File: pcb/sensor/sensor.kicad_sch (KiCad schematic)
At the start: 53 parts, among them J3 sig_in, J4 sig_out, J7 Conn_02x02_Counter_Clockwise, SW2 SW_SPST, U1 SIT1042AQT/3, U2 HX711, U5 LMR16030SDDAR, U8 LMR16030SDDAR, U9 LMR16030SDDAR

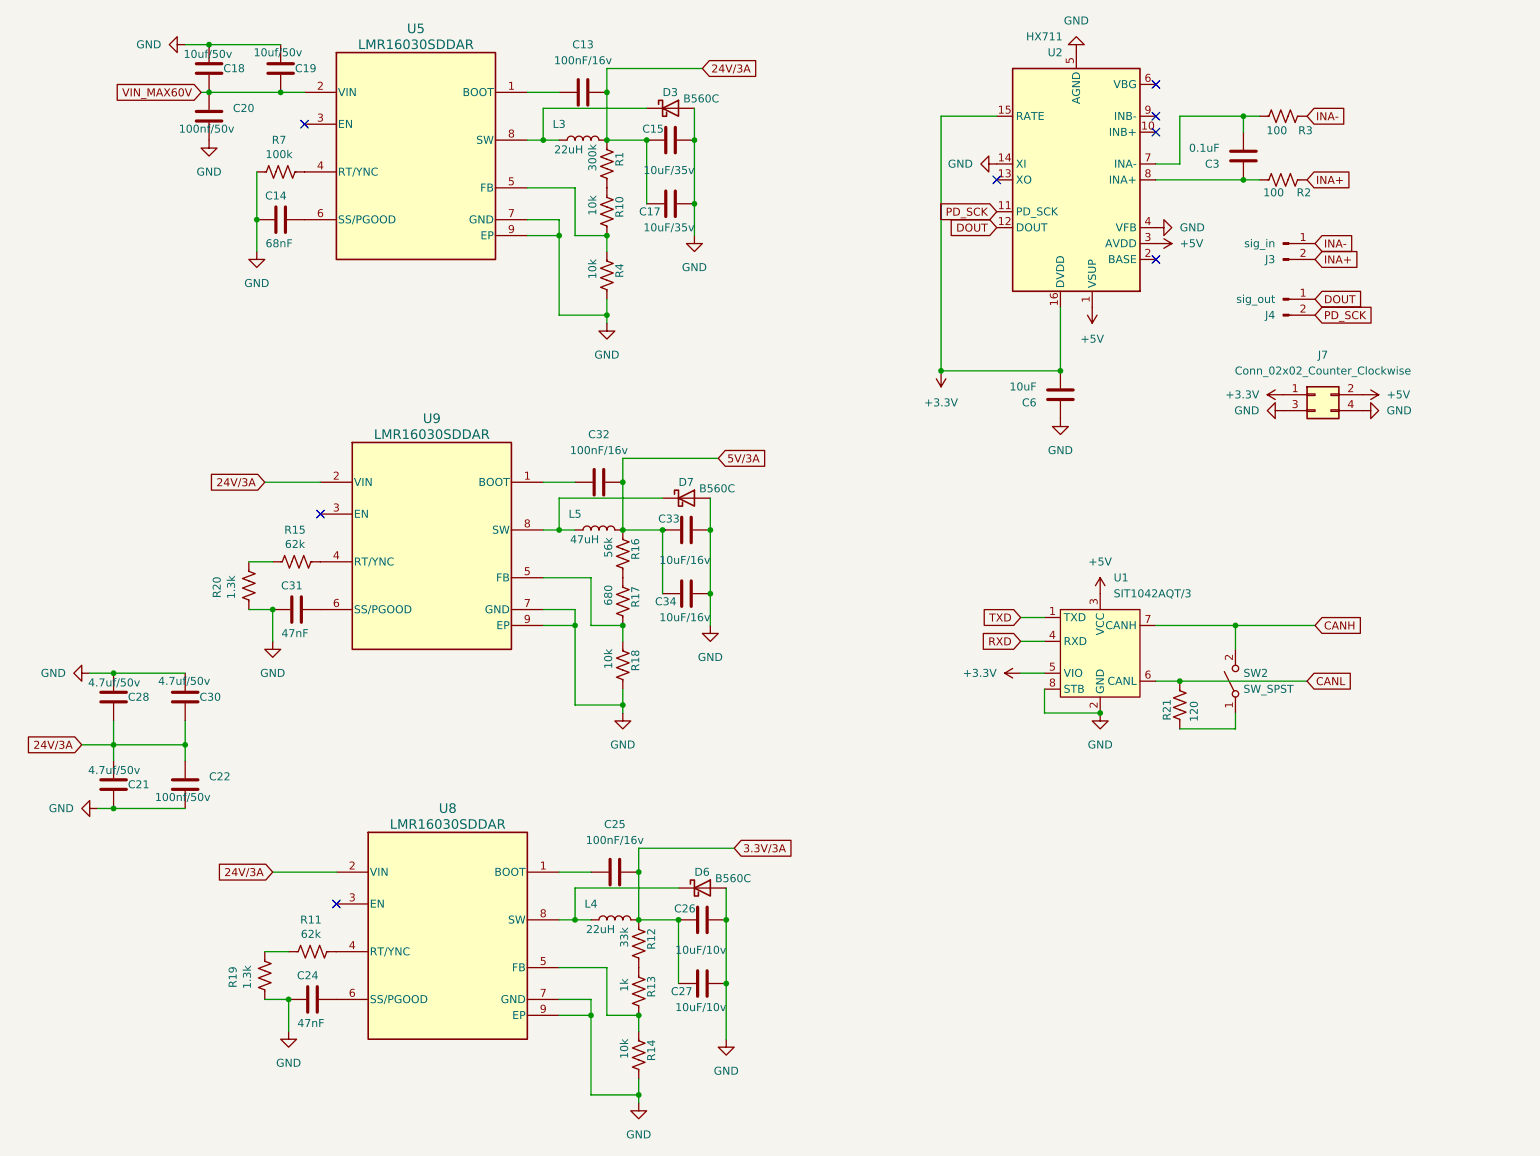
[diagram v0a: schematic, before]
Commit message: feat: update
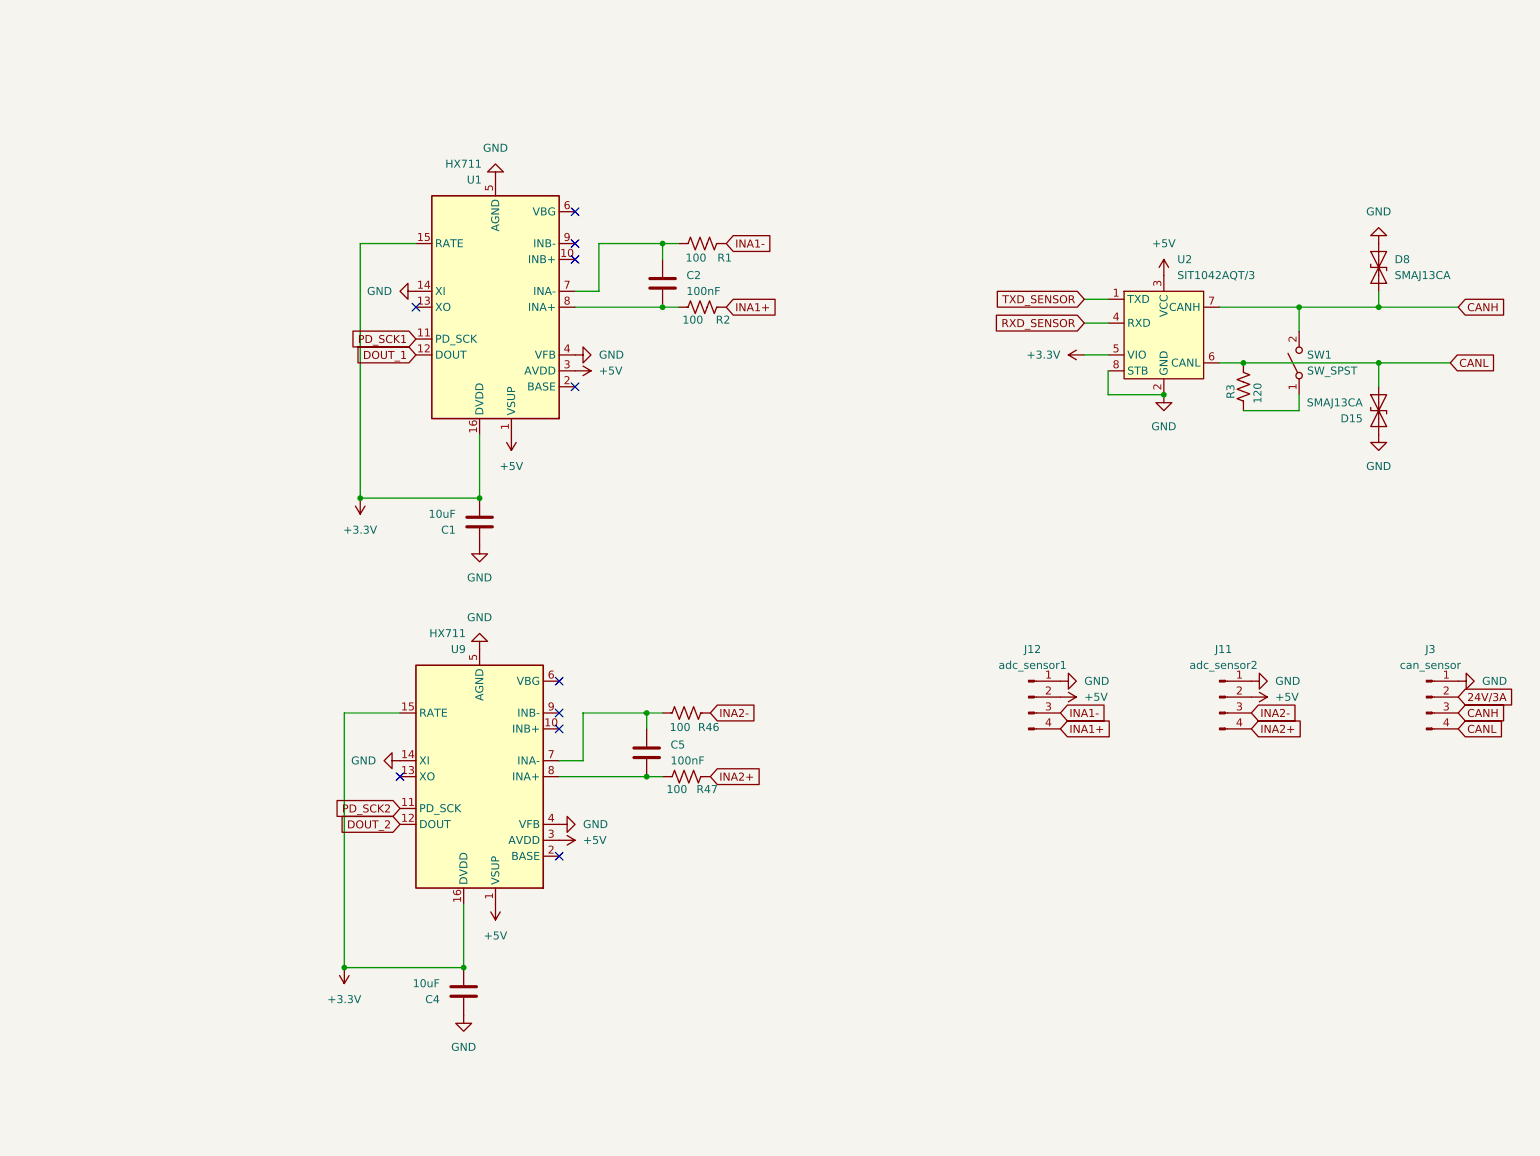
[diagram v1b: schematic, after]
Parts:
- removed C13, C25, C32: 100nF/16v, Capacitor_SMD:C_0603_1608Metric, symbol Device:C
- removed C14: 68nF, Capacitor_SMD:C_0603_1608Metric, symbol Device:C
- removed C15, C17: 10uF/35v, Capacitor_SMD:C_1210_3225Metric, symbol Device:C
- removed C18, C19: 10uf/50v, Capacitor_SMD:C_1210_3225Metric, symbol Device:C
- removed C20, C22: 100nf/50v, Capacitor_SMD:C_0603_1608Metric, symbol Device:C
- removed C21, C28, C30: 4.7uf/50v, Capacitor_SMD:C_1206_3216Metric, symbol Device:C
- removed C24, C31: 47nF, Capacitor_SMD:C_0603_1608Metric, symbol Device:C
- removed C26, C27: 10uF/10v, Capacitor_SMD:C_0603_1608Metric, symbol Device:C
- removed C33, C34: 10uF/16v, Capacitor_SMD:C_1210_3225Metric, symbol Device:C
- removed D3, D6, D7: B560C, Diode_SMD:D_SMC, symbol Device:D_Schottky
- removed J3: sig_in, Connector_PinHeader_2.54mm:PinHeader_1x02_P2.54mm_Vertical, symbol Connector:Conn_01x02_Pin
- removed J4: sig_out, Connector_PinHeader_2.54mm:PinHeader_1x02_P2.54mm_Vertical, symbol Connector:Conn_01x02_Pin
- removed J7: Conn_02x02_Counter_Clockwise, Connector_PinHeader_2.54mm:PinHeader_2x02_P2.54mm_Vertical, symbol Connector_Generic:Conn_02x02_Odd_Even
- removed L3, L4: 22uH, Inductor_SMD:L_TDK_SLF12565, symbol Device:L
- removed L5: 47uH, Inductor_SMD:L_TDK_SLF12565, symbol Device:L
- removed R1: 300k, Resistor_SMD:R_0603_1608Metric, symbol Device:R_US
- removed R10, R14, R18, R4: 10k, Resistor_SMD:R_0603_1608Metric, symbol Device:R_US
- removed R11, R15: 62k, Resistor_SMD:R_0603_1608Metric, symbol Device:R_US
- removed R12: 33k, Resistor_SMD:R_0603_1608Metric, symbol Device:R_US
- removed R13: 1k, Resistor_SMD:R_0603_1608Metric, symbol Device:R_US
- removed R16: 56k, Resistor_SMD:R_0603_1608Metric, symbol Device:R_US
- removed R17: 680, Resistor_SMD:R_0603_1608Metric, symbol Device:R_US
- removed R19, R20: 1.3k, Resistor_SMD:R_0603_1608Metric, symbol Device:R_US
- removed R7: 100k, Resistor_SMD:R_0603_1608Metric, symbol Device:R_US
- removed U5, U8, U9: LMR16030SDDAR, Package_SO:TI_SO-PowerPAD-8_ThermalVias, symbol 2025-01-08_11-11-09:LMR16030SDDAR
- added C4: 10uF, Capacitor_SMD:C_0603_1608Metric, symbol Device:C
- added C5: 100nF, Capacitor_SMD:C_0603_1608Metric, symbol Device:C
- added D15, D8: SMAJ13CA, Diode_SMD:D_SMA, symbol Diode:SMAJ13CA
- added J11: adc_sensor2, TerminalBlock:TerminalBlock_MaiXu_MX126-5.0-04P_1x04_P5.00mm, symbol Connector:Conn_01x04_Pin
- added J12: adc_sensor1, TerminalBlock:TerminalBlock_MaiXu_MX126-5.0-04P_1x04_P5.00mm, symbol Connector:Conn_01x04_Pin
- added J3: can_sensor, TerminalBlock:TerminalBlock_MaiXu_MX126-5.0-04P_1x04_P5.00mm, symbol Connector:Conn_01x04_Pin
- added R46, R47: 100, Resistor_SMD:R_0603_1608Metric, symbol Device:R_US
- added U9: HX711, Package_SO:SOP-16_3.9x9.9mm_P1.27mm, symbol Analog_ADC:HX711
- C2: renamed from C3; value 0.1uF -> 100nF
- renumbered C6 to C1, R3 to R1, R21 to R3, SW2 to SW1, U2 to U1, U1 to U2
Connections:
- net +3.3V: now also C4.2, U9.15 (RATE), U9.16 (DVDD)
- net +5V: now also J11.2 (Pin_2), J12.2 (Pin_2), U9.1 (VSUP), U9.3 (AVDD)
- net 24V/3A: now also J3.2 (Pin_2)
- net CANH: now also D8.1 (A1), J3.3 (Pin_3)
- net CANL: now also D15.1 (A1), J3.4 (Pin_4)
- net GND: now also C4.1, D15.2 (A2), D8.2 (A2), J11.1 (Pin_1), J12.1 (Pin_1), J3.1 (Pin_1), U9.14 (XI), U9.4 (VFB), U9.5 (AGND)
- net DOUT renamed DOUT_1
- net INA+ renamed INA1+
- net INA1+: now also J12.4 (Pin_4)
- net INA- renamed INA1-
- net INA1-: now also J12.3 (Pin_3)
- net PD_SCK renamed PD_SCK1
- net RXD renamed RXD_SENSOR
- net TXD renamed TXD_SENSOR
- new net: C5.1, R47.1, U9.8 (INA+)
- new net: C5.2, R46.1, U9.7 (INA-)
- new net DOUT_2: U9.12 (DOUT)
- new net INA2+: J11.4 (Pin_4), R47.2
- new net INA2-: J11.3 (Pin_3), R46.2
- new net PD_SCK2: U9.11 (PD_SCK)
- no-connect marks 8 -> 10
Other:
- moved on the sheet: C1, C2, R1, R2, R3, SW1, U1, U2

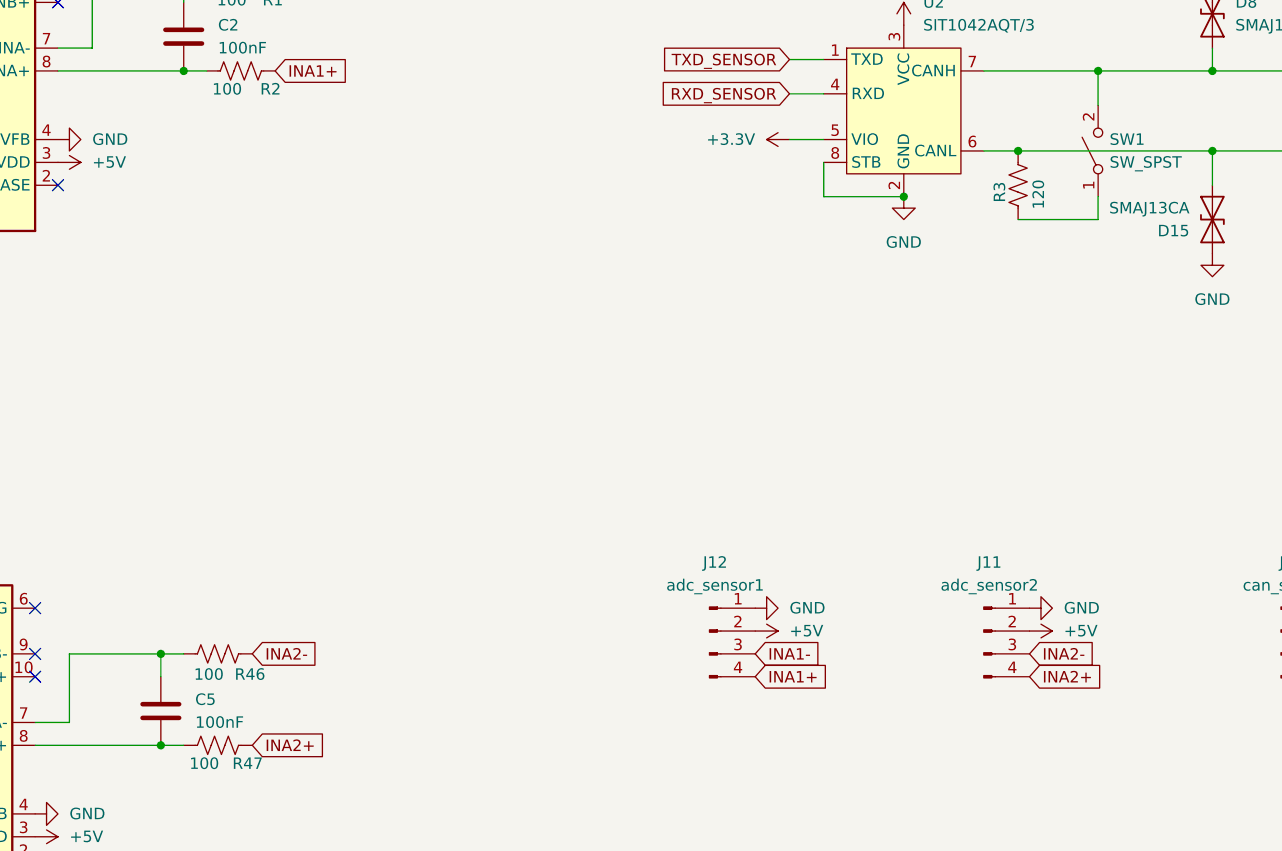
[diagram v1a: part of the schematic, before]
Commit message: feat: update
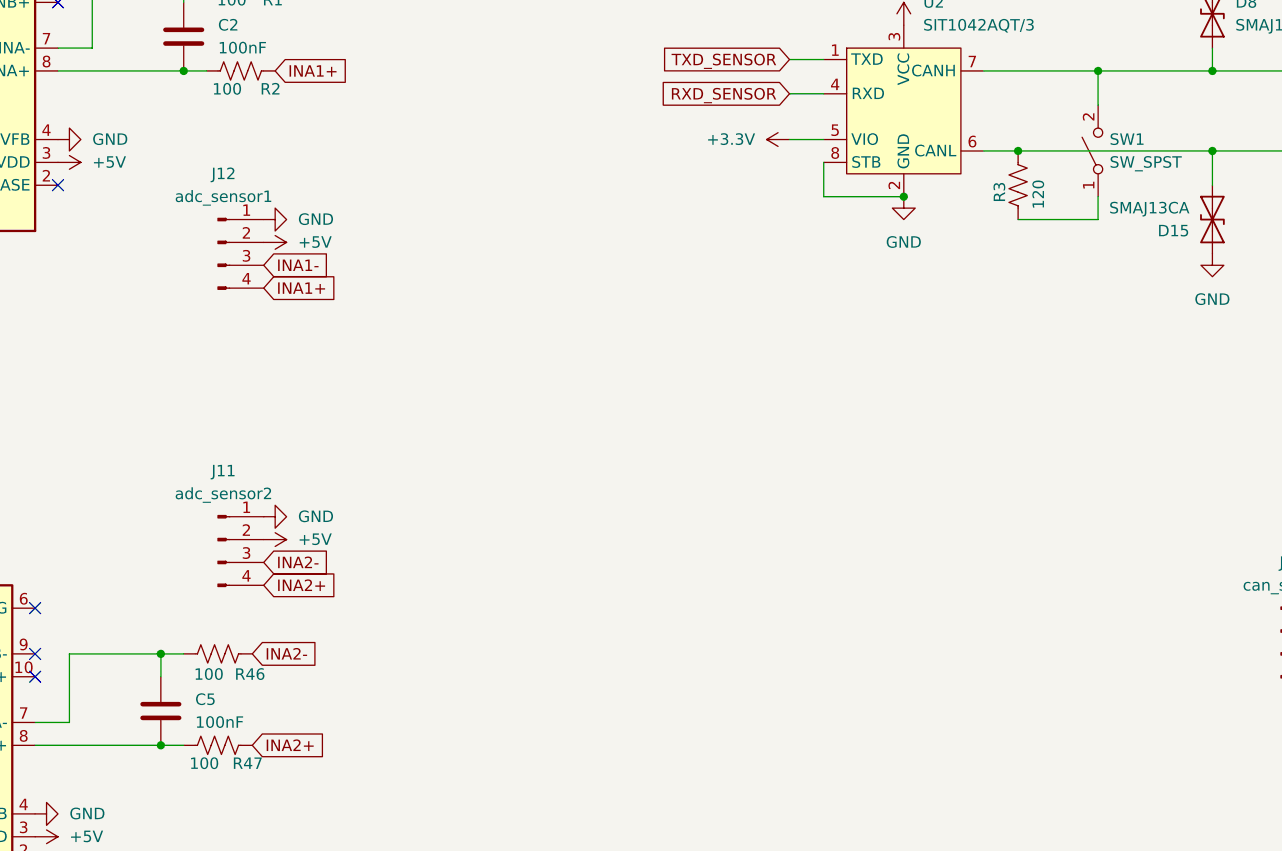
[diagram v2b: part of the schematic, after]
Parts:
- J11, J12, J3: footprint TerminalBlock:TerminalBlock_MaiXu_MX126-5.0-04P_1x04_P5.00mm -> Connector_JST:JST_PH_B4B-PH-K_1x04_P2.00mm_Vertical
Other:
- moved on the sheet: J11, J12
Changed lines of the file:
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@@
 	(global_label "INA2+"
 		(shape input)
-		(at 217.17 132.08 0)
+		(at 132.08 121.92 0)
 		(fields_autoplaced yes)
 		(effects
@@
 		)
 		(property "Intersheetrefs" "${INTERSHEET_REFS}"
-			(at 225.961 132.08 0)
+			(at 140.871 121.92 0)
 			(hide yes)
 			(effects
@@
 	(global_label "INA1+"
 		(shape input)
-		(at 186.69 132.08 0)
+		(at 132.08 88.9 0)
 		(fields_autoplaced yes)
 		(effects
@@
 		)
 		(property "Intersheetrefs" "${INTERSHEET_REFS}"
-			(at 195.481 132.08 0)
+			(at 140.871 88.9 0)
 			(hide yes)
 			(effects
@@
 	(global_label "INA1-"
 		(shape input)
-		(at 186.69 129.54 0)
+		(at 132.08 86.36 0)
 		(fields_autoplaced yes)
 		(effects
@@
 		)
 		(property "Intersheetrefs" "${INTERSHEET_REFS}"
-			(at 195.481 129.54 0)
+			(at 140.871 86.36 0)
 			(hide yes)
 			(effects
@@
 	(global_label "INA2-"
 		(shape input)
-		(at 217.17 129.54 0)
+		(at 132.08 119.38 0)
 		(fields_autoplaced yes)
 		(effects
@@
 		)
 		(property "Intersheetrefs" "${INTERSHEET_REFS}"
-			(at 225.961 129.54 0)
+			(at 140.871 119.38 0)
 			(hide yes)
 			(effects
@@
 	(symbol
 		(lib_id "power:+5V")
-		(at 217.17 127 270)
+		(at 132.08 116.84 270)
 		(unit 1)
 		(exclude_from_sim no)
@@
 		(fields_autoplaced yes)
 		(property "Reference" "#PWR0142"
-			(at 213.36 127 0)
+			(at 128.27 116.84 0)
 			(hide yes)
 			(effects
@@
 		)
 		(property "Value" "+5V"
-			(at 220.98 126.9999 90)
+			(at 135.89 116.8399 90)
 			(effects
 				(font
@@
 		)
 		(property "Footprint" ""
-			(at 217.17 127 0)
+			(at 132.08 116.84 0)
 			(hide yes)
 			(effects
@@
 		)
 		(property "Datasheet" ""
-			(at 217.17 127 0)
+			(at 132.08 116.84 0)
 			(hide yes)
 			(effects
@@
 		)
 		(property "Description" "Power symbol creates a global label with name \"+5V\""
-			(at 217.17 127 0)
+			(at 132.08 116.84 0)
 			(hide yes)
 			(effects
@@
 	(symbol
 		(lib_id "Connector:Conn_01x04_Pin")
-		(at 212.09 127 0)
+		(at 127 116.84 0)
 		(unit 1)
 		(exclude_from_sim no)
@@
 		(fields_autoplaced yes)
 		(property "Reference" "J11"
-			(at 212.725 119.38 0)
+			(at 127.635 109.22 0)
 			(effects
 				(font
@@
 		)
 		(property "Value" "adc_sensor2"
-			(at 212.725 121.92 0)
-			(effects
-				(font
-					(size 1.27 1.27)
-				)
-			)
-		)
-		(property "Footprint" "TerminalBlock:TerminalBlock_MaiXu_MX126-5.0-04P_1x04_P5.00mm"
-			(at 212.09 127 0)
+			(at 127.635 111.76 0)
+			(effects
+				(font
+					(size 1.27 1.27)
+				)
+			)
+		)
+		(property "Footprint" "Connector_JST:JST_PH_B4B-PH-K_1x04_P2.00mm_Vertical"
+			(at 127 116.84 0)
 			(hide yes)
 			(effects
@@
 		)
 		(property "Datasheet" "~"
-			(at 212.09 127 0)
+			(at 127 116.84 0)
 			(hide yes)
 			(effects
@@
 		)
 		(property "Description" "Generic connector, single row, 01x04, script generated"
-			(at 212.09 127 0)
+			(at 127 116.84 0)
 			(hide yes)
 			(effects
@@
 	(symbol
 		(lib_id "Connector:Conn_01x04_Pin")
-		(at 181.61 127 0)
+		(at 127 83.82 0)
 		(unit 1)
 		(exclude_from_sim no)
@@
 		(fields_autoplaced yes)
 		(property "Reference" "J12"
-			(at 182.245 119.38 0)
+			(at 127.635 76.2 0)
 			(effects
 				(font
@@
 		)
 		(property "Value" "adc_sensor1"
-			(at 182.245 121.92 0)
-			(effects
-				(font
-					(size 1.27 1.27)
-				)
-			)
-		)
-		(property "Footprint" "TerminalBlock:TerminalBlock_MaiXu_MX126-5.0-04P_1x04_P5.00mm"
-			(at 181.61 127 0)
+			(at 127.635 78.74 0)
+			(effects
+				(font
+					(size 1.27 1.27)
+				)
+			)
+		)
+		(property "Footprint" "Connector_JST:JST_PH_B4B-PH-K_1x04_P2.00mm_Vertical"
+			(at 127 83.82 0)
 			(hide yes)
 			(effects
@@
 		)
 		(property "Datasheet" "~"
-			(at 181.61 127 0)
+			(at 127 83.82 0)
 			(hide yes)
 			(effects
@@
 		)
 		(property "Description" "Generic connector, single row, 01x04, script generated"
-			(at 181.61 127 0)
+			(at 127 83.82 0)
 			(hide yes)
 			(effects
@@
 			)
 		)
-		(property "Footprint" "TerminalBlock:TerminalBlock_MaiXu_MX126-5.0-04P_1x04_P5.00mm"
+		(property "Footprint" "Connector_JST:JST_PH_B4B-PH-K_1x04_P2.00mm_Vertical"
 			(at 245.11 127 0)
 			(hide yes)
@@
 	(symbol
 		(lib_id "power:+5V")
-		(at 186.69 127 270)
+		(at 132.08 83.82 270)
 		(unit 1)
 		(exclude_from_sim no)
@@
 		(fields_autoplaced yes)
 		(property "Reference" "#PWR0107"
-			(at 182.88 127 0)
+			(at 128.27 83.82 0)
 			(hide yes)
 			(effects
@@
 		)
 		(property "Value" "+5V"
-			(at 190.5 126.9999 90)
+			(at 135.89 83.8199 90)
 			(effects
 				(font
@@
 		)
 		(property "Footprint" ""
-			(at 186.69 127 0)
+			(at 132.08 83.82 0)
 			(hide yes)
 			(effects
@@
 		)
 		(property "Datasheet" ""
-			(at 186.69 127 0)
+			(at 132.08 83.82 0)
 			(hide yes)
 			(effects
@@
 		)
 		(property "Description" "Power symbol creates a global label with name \"+5V\""
-			(at 186.69 127 0)
+			(at 132.08 83.82 0)
 			(hide yes)
 			(effects
@@
 	(symbol
 		(lib_id "power:GND")
-		(at 217.17 124.46 90)
+		(at 132.08 114.3 90)
 		(unit 1)
 		(exclude_from_sim no)
@@
 		(fields_autoplaced yes)
 		(property "Reference" "#PWR0105"
-			(at 223.52 124.46 0)
+			(at 138.43 114.3 0)
 			(hide yes)
 			(effects
@@
 		)
 		(property "Value" "GND"
-			(at 220.98 124.4601 90)
+			(at 135.89 114.3001 90)
 			(effects
 				(font
@@
 		)
 		(property "Footprint" ""
-			(at 217.17 124.46 0)
+			(at 132.08 114.3 0)
 			(hide yes)
 			(effects
@@
 		)
 		(property "Datasheet" ""
-			(at 217.17 124.46 0)
+			(at 132.08 114.3 0)
 			(hide yes)
 			(effects
@@
 		)
 		(property "Description" "Power symbol creates a global label with name \"GND\" , ground"
-			(at 217.17 124.46 0)
+			(at 132.08 114.3 0)
 			(hide yes)
 			(effects
@@
 	(symbol
 		(lib_id "power:GND")
-		(at 186.69 124.46 90)
+		(at 132.08 81.28 90)
 		(unit 1)
 		(exclude_from_sim no)
@@
 		(fields_autoplaced yes)
 		(property "Reference" "#PWR0106"
-			(at 193.04 124.46 0)
+			(at 138.43 81.28 0)
 			(hide yes)
 			(effects
@@
 		)
 		(property "Value" "GND"
-			(at 190.5 124.4601 90)
+			(at 135.89 81.2801 90)
 			(effects
 				(font
@@
 		)
 		(property "Footprint" ""
-			(at 186.69 124.46 0)
+			(at 132.08 81.28 0)
 			(hide yes)
 			(effects
@@
 		)
 		(property "Datasheet" ""
-			(at 186.69 124.46 0)
+			(at 132.08 81.28 0)
 			(hide yes)
 			(effects
@@
 		)
 		(property "Description" "Power symbol creates a global label with name \"GND\" , ground"
-			(at 186.69 124.46 0)
-			(hide yes)
-			(effects
+			(at 132.08 81.28 0)
+			(hide yes)
+			(effects
